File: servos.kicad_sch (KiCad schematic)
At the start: 33 parts, among them J10 Conn_01x03, J11 Conn_01x03, J6 Conn_01x03, J7 Conn_01x03, J8 Conn_01x03, J9 Conn_01x03, U10 INA745A, U11 INA745A, U12 INA745A, U13 INA745A, U6 INA745A, U9 INA745A

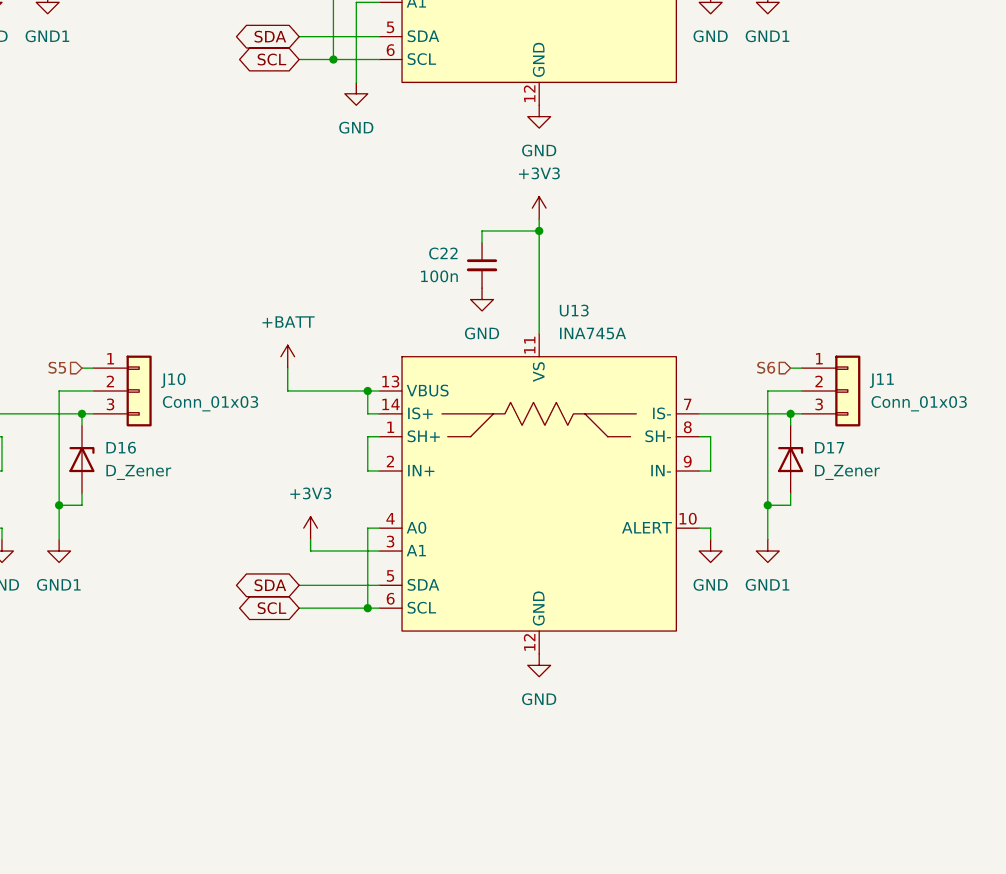
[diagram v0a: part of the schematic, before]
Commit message: remove unneeded stuff
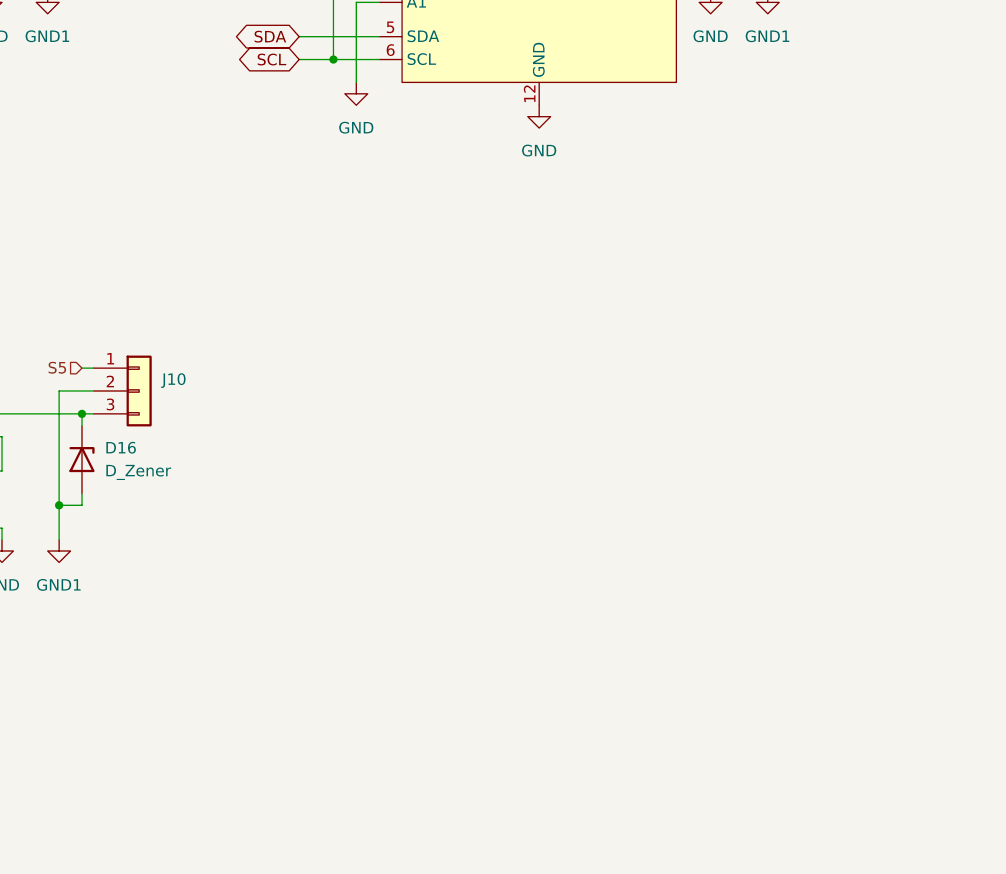
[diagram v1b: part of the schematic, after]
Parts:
- removed C22: 100n, Capacitor_SMD:C_0402_1005Metric, symbol Device:C_Small
- removed D17: D_Zener, Diode_SMD:Nexperia_CFP3_SOD-123W, symbol Device:D_Zener
- removed J11: Conn_01x03, beavs-footprints:JST_VH_B3P-VH-B_1x03_P3.96mm_Vertical_model, symbol Connector_Generic:Conn_01x03
- removed U13: INA745A, beavs-footprints:QFN-14-REL_TI, symbol beavs-symbols:INA745
